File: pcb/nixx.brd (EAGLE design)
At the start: 20 x 40 mm, 44 parts, among them IC1 24C64ST

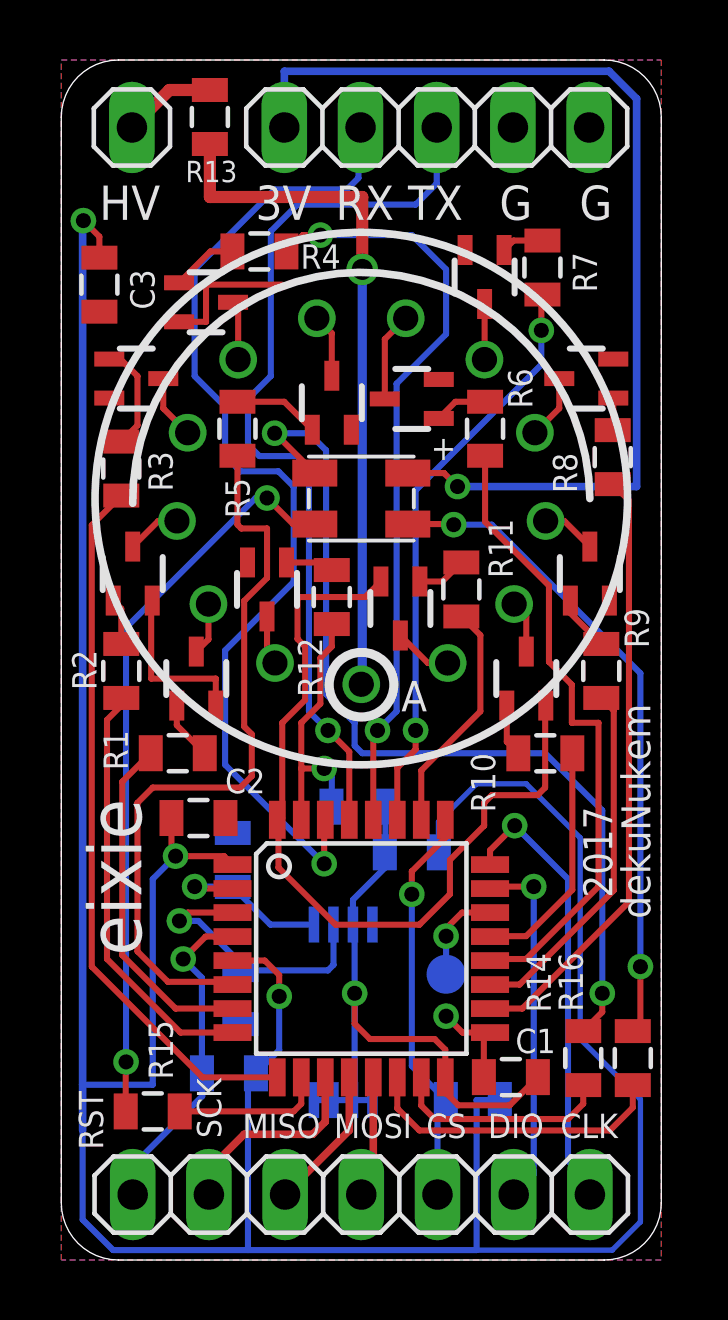
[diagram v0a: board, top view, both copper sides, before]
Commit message: USBC, GPS etc
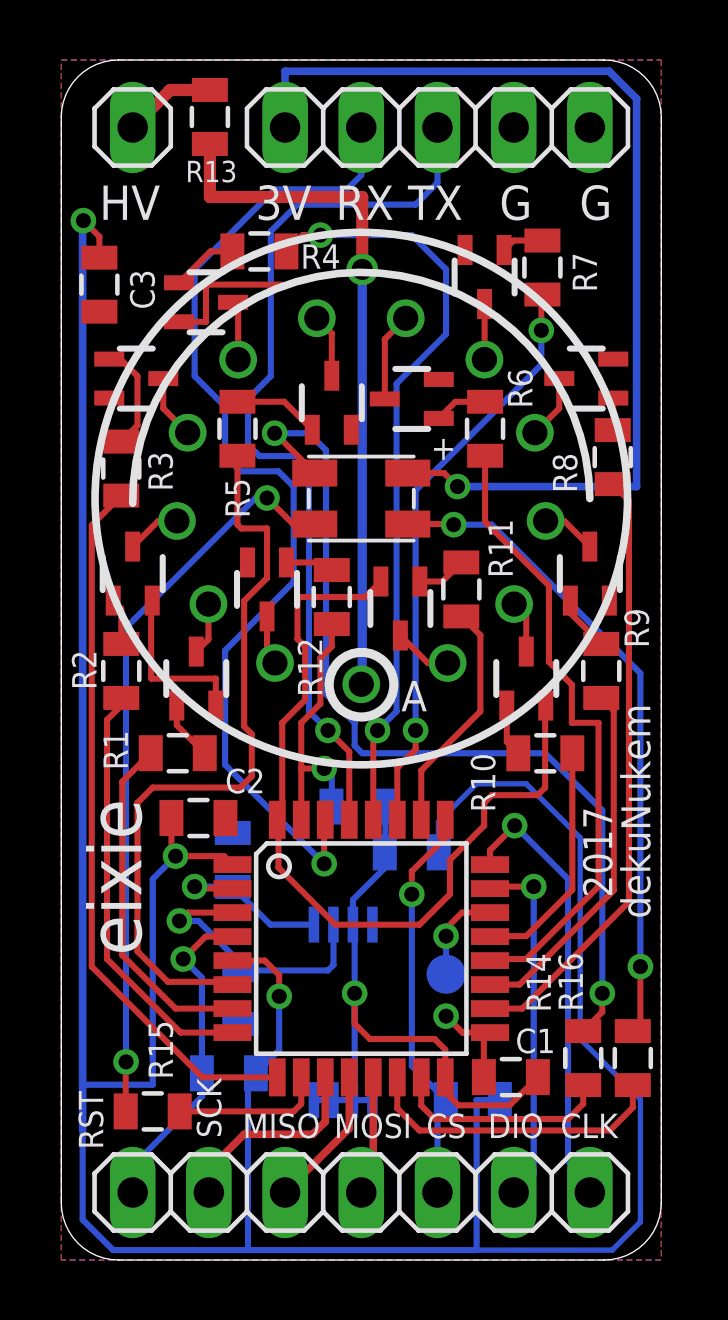
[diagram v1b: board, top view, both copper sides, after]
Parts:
- moved JP2 0.07 mm to (10.0, 2.25)
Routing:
- net SPI_SCK: track 6.85 -> 5.97 mm
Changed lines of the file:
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@@
 <grid distance="5" unitdist="mil" unit="mil" style="lines" multiple="1" display="no" altdistance="1" altunitdist="mil" altunit="mil"/>
 <layers>
-<layer number="1" name="Top" color="4" fill="1" visible="no" active="yes"/>
+<layer number="1" name="Top" color="4" fill="1" visible="yes" active="yes"/>
 <layer number="16" name="Bottom" color="1" fill="1" visible="yes" active="yes"/>
 <layer number="17" name="Pads" color="2" fill="1" visible="yes" active="yes"/>
@@
 <layer number="20" name="Dimension" color="15" fill="1" visible="yes" active="yes"/>
 <layer number="21" name="tPlace" color="7" fill="1" visible="no" active="yes"/>
-<layer number="22" name="bPlace" color="7" fill="1" visible="yes" active="yes"/>
-<layer number="23" name="tOrigins" color="15" fill="1" visible="no" active="yes"/>
-<layer number="24" name="bOrigins" color="15" fill="1" visible="yes" active="yes"/>
+<layer number="22" name="bPlace" color="7" fill="1" visible="no" active="yes"/>
+<layer number="23" name="tOrigins" color="15" fill="1" visible="yes" active="yes"/>
+<layer number="24" name="bOrigins" color="15" fill="1" visible="no" active="yes"/>
 <layer number="25" name="tNames" color="7" fill="1" visible="no" active="yes"/>
-<layer number="26" name="bNames" color="7" fill="1" visible="yes" active="yes"/>
+<layer number="26" name="bNames" color="7" fill="1" visible="no" active="yes"/>
 <layer number="27" name="tValues" color="7" fill="1" visible="no" active="yes"/>
 <layer number="28" name="bValues" color="7" fill="1" visible="no" active="yes"/>
@@
 <element name="N1" library="russian-nixies" package="IN-14" value="IN-14" x="10" y="25.381" smashed="yes"/>
 <element name="U$2" library="nixx" package="TQFP32-08" value="STM32F042K6" x="10" y="10.381" smashed="yes"/>
-<element name="JP2" library="pinhead" package="1X07" value="" x="10" y="2.181" smashed="yes">
-<attribute name="VALUE" x="1.11" y="-0.994" size="1.27" layer="27"/>
+<element name="JP2" library="pinhead" package="1X07" value="" x="10" y="2.25" smashed="yes">
+<attribute name="VALUE" x="1.11" y="-0.925" size="1.27" layer="27"/>
 </element>
 <element name="Q1" library="nixx" package="SOT323" value="" x="4.5" y="19.381" smashed="yes">
@@
 <attribute name="NAME" x="2.2987" y="33.02" size="0.8128" layer="25" font="vector" rot="R270"/>
 </element>
-<element name="JP1" library="nixx" package="1X07" value="" x="9.9746" y="37.7508" smashed="yes">
-<attribute name="VALUE" x="1.0846" y="34.5758" size="1.27" layer="27"/>
+<element name="JP1" library="nixx" package="1X07" value="" x="10" y="37.75" smashed="yes">
+<attribute name="VALUE" x="1.11" y="34.575" size="1.27" layer="27"/>
 </element>
 <element name="D1" library="nixx" package="3528-COMMON-ANODE" value="RGB_LED_CA-150141M173100-R&amp;G&amp;B" x="10" y="25.381" smashed="yes"/>
@@
 <wire x1="14.2926" y1="7.581" x2="13.374" y2="7.581" width="0.2032" layer="1"/>
 <wire x1="13.374" y1="7.581" x2="12.827" y2="8.128" width="0.2032" layer="1"/>
-<wire x1="7.4346" y1="37.7508" x2="7.4346" y2="39.624" width="0.254" layer="16"/>
-<wire x1="7.4346" y1="39.624" x2="18.2626" y2="39.624" width="0.254" layer="16"/>
 <wire x1="18.2626" y1="39.624" x2="19.177" y2="38.7096" width="0.254" layer="16"/>
 <wire x1="19.177" y1="38.7096" x2="19.177" y2="25.781" width="0.254" layer="16"/>
@@
 <wire x1="19.304" y1="1.27" x2="19.304" y2="5.3594" width="0.1778" layer="16"/>
 <wire x1="19.304" y1="5.3594" x2="17.2974" y2="7.366" width="0.1778" layer="16"/>
+<wire x1="7.46" y1="37.75" x2="7.46" y2="39.624" width="0.254" layer="16"/>
+<wire x1="7.46" y1="39.624" x2="18.2626" y2="39.624" width="0.254" layer="16"/>
 </signal>
 <signal name="SPI_SCK">
@@
 <wire x1="8.382" y1="4.191" x2="6.096" y2="4.191" width="0.254" layer="1"/>
 <wire x1="6.096" y1="4.191" x2="4.953" y2="3.048" width="0.254" layer="1"/>
-<wire x1="4.953" y1="3.048" x2="4.953" y2="2.214" width="0.254" layer="1"/>
-<wire x1="4.953" y1="2.214" x2="4.92" y2="2.181" width="0.254" layer="1"/>
+<wire x1="4.92" y1="2.25" x2="4.953" y2="3.048" width="0" layer="19" extent="1-1"/>
 </signal>
 <signal name="SPI_MISO">
 <contactref element="JP2" pad="3"/>
 <contactref element="U$2" pad="12"/>
-<wire x1="9.6" y1="6.0884" x2="9.6" y2="4.321" width="0.254" layer="1"/>
-<wire x1="9.6" y1="4.321" x2="7.46" y2="2.181" width="0.254" layer="1"/>
+<wire x1="9.6" y1="6.0884" x2="9.6" y2="4.39" width="0.254" layer="1"/>
+<wire x1="9.6" y1="4.39" x2="7.46" y2="2.25" width="0.254" layer="1"/>
 </signal>
 <signal name="SPI_MOSI">
 <contactref element="JP2" pad="4"/>
 <contactref element="U$2" pad="13"/>
-<wire x1="10.4" y1="6.0884" x2="10.4" y2="2.581" width="0.254" layer="1"/>
-<wire x1="10.4" y1="2.581" x2="10" y2="2.181" width="0.254" layer="1"/>
+<wire x1="10.4" y1="6.0884" x2="10.4" y2="2.65" width="0.254" layer="1"/>
+<wire x1="10.4" y1="2.65" x2="10" y2="2.25" width="0.254" layer="1"/>
 </signal>
 <signal name="SPI_CS">
@@
 <wire x1="11.684" y1="12.192" x2="11.684" y2="6.466" width="0.2032" layer="16"/>
 <wire x1="11.684" y1="6.466" x2="12.816" y2="5.334" width="0.2032" layer="16"/>
-<wire x1="12.54" y1="2.181" x2="12.54" y2="5.058" width="0.2032" layer="16"/>
+<wire x1="12.54" y1="2.25" x2="12.54" y2="5.058" width="0.2032" layer="16"/>
 <wire x1="12.54" y1="5.058" x2="12.816" y2="5.334" width="0.2032" layer="16"/>
 <contactref element="U$2" pad="25"/>
@@
 <via x="15.748" y="12.446" extent="1-16" drill="0.5"/>
 <wire x1="15.748" y1="12.446" x2="15.748" y2="2.849" width="0.2032" layer="16"/>
-<wire x1="15.748" y1="2.849" x2="15.08" y2="2.181" width="0.2032" layer="16"/>
+<wire x1="15.748" y1="2.849" x2="15.149" y2="2.25" width="0.2032" layer="16"/>
+<wire x1="15.149" y1="2.25" x2="15.08" y2="2.25" width="0.2032" layer="16"/>
 </signal>
 <signal name="SWD_CLK">
@@
 <wire x1="16.891" y1="12.7" x2="16.891" y2="3.302" width="0.2032" layer="16"/>
 <wire x1="16.891" y1="3.302" x2="17.62" y2="2.573" width="0.2032" layer="16"/>
-<wire x1="17.62" y1="2.573" x2="17.62" y2="2.181" width="0.2032" layer="16"/>
+<wire x1="17.62" y1="2.573" x2="17.62" y2="2.25" width="0.2032" layer="16"/>
 </signal>
 <signal name="NRST">
@@
 <wire x1="4.812" y1="10.781" x2="4.064" y2="10.033" width="0.2032" layer="1"/>
 <wire x1="4.688" y1="9.409" x2="4.064" y2="10.033" width="0.2032" layer="16"/>
-<wire x1="2.38" y1="2.181" x2="2.38" y2="3.142" width="0.2032" layer="16"/>
+<wire x1="2.38" y1="2.25" x2="2.38" y2="3.142" width="0.2032" layer="16"/>
 <wire x1="2.38" y1="3.142" x2="4.699" y2="5.461" width="0.2032" layer="16"/>
 <wire x1="4.699" y1="5.461" x2="4.699" y2="6.212" width="0.2032" layer="16"/>
@@
 <wire x1="4.445" y1="29.464" x2="4.445" y2="33.02" width="0.2032" layer="16"/>
 <wire x1="7.112" y1="35.687" x2="9.525" y2="35.687" width="0.2032" layer="16"/>
-<wire x1="9.525" y1="35.687" x2="9.906" y2="36.068" width="0.2032" layer="16"/>
-<wire x1="9.906" y1="36.068" x2="9.906" y2="37.6822" width="0.2032" layer="16"/>
-<wire x1="9.906" y1="37.6822" x2="9.9746" y2="37.7508" width="0.2032" layer="16"/>
 <wire x1="7.112" y1="35.687" x2="4.445" y2="33.02" width="0.2032" layer="16"/>
+<wire x1="9.525" y1="35.687" x2="10" y2="36.162" width="0.2032" layer="16"/>
+<wire x1="10" y1="36.162" x2="10" y2="37.75" width="0.2032" layer="16"/>
 </signal>
 <signal name="UART_TX">
@@
 <wire x1="6.985" y1="34.29" x2="7.874" y2="35.179" width="0.2032" layer="16"/>
 <wire x1="7.874" y1="35.179" x2="11.811" y2="35.179" width="0.2032" layer="16"/>
-<wire x1="11.811" y1="35.179" x2="12.5146" y2="35.8826" width="0.2032" layer="16"/>
-<wire x1="12.5146" y1="35.8826" x2="12.5146" y2="37.7508" width="0.2032" layer="16"/>
 <wire x1="9.6" y1="14.6736" x2="9.6" y2="16.943" width="0.2032" layer="1"/>
 <wire x1="9.6" y1="16.943" x2="8.89" y2="17.653" width="0.2032" layer="1"/>
 <wire x1="8.89" y1="17.653" x2="8.255" y2="18.288" width="0.2032" layer="16"/>
 <wire x1="8.255" y1="18.288" x2="8.255" y2="26.416" width="0.2032" layer="16"/>
+<wire x1="11.811" y1="35.179" x2="12.54" y2="35.908" width="0.2032" layer="16"/>
+<wire x1="12.54" y1="35.908" x2="12.54" y2="37.75" width="0.2032" layer="16"/>
 </signal>
 <signal name="N$2">
 <contactref element="JP1" pad="1"/>
 <contactref element="R13" pad="2"/>
-<wire x1="2.3546" y1="37.7508" x2="3.6038" y2="39" width="0.4064" layer="1"/>
-<wire x1="3.6038" y1="39" x2="4.953" y2="39" width="0.4064" layer="1"/>
+<wire x1="2.38" y1="37.75" x2="3.63" y2="39" width="0.4064" layer="1"/>
+<wire x1="3.63" y1="39" x2="4.953" y2="39" width="0.4064" layer="1"/>
 </signal>
 <signal name="STM_DOT_LEFT">
